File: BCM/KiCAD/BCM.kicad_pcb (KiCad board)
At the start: 2 copper layers, 150 x 99.1 mm, 157 parts, among them J10 Back_9, J11 Back_10, J12 Back_11, J13 Back_12, J14 Eye1, J15 Eye2, J16 Nose, J17 S1, J18 S2, J19 S3, J2 Back_1, J20 S4, J21 S5, J22 Door2, J23 Door1, J24 But1, J25 But2, J26 But3, J27 But4, J28 But5, J29 But6, J3 Back_2, J30 Power, J4 Back_3, J5 Back_4, J6 Back_5, J7 Back_6, J8 Back_7, J9 Back_8, Q1 2N7002, Q10 2N7002, Q11 2N7002, Q12 2N7002, Q13 2N7002, Q14 2N7002, Q15 2N7002, Q16 2N7002, Q17 2N7002, Q18 2N7002, Q19 2N7002, Q2 2N7002, Q20 2N7002, Q3 2N7002, Q4 2N7002, Q5 2N7002, Q6 2N7002, Q7 2N7002, Q8 2N7002, Q9 2N7002, U1 TPS54331D

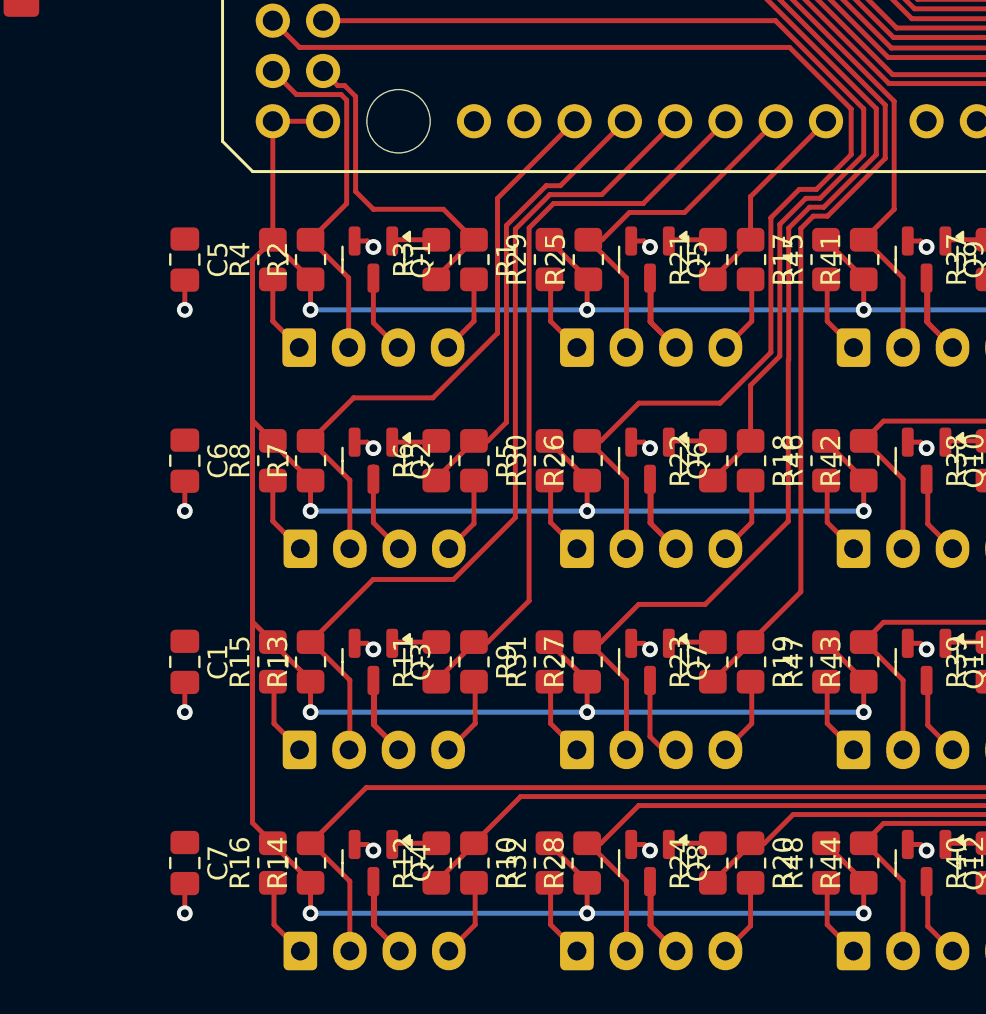
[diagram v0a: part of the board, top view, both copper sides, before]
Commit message: move buttons to own supply rail
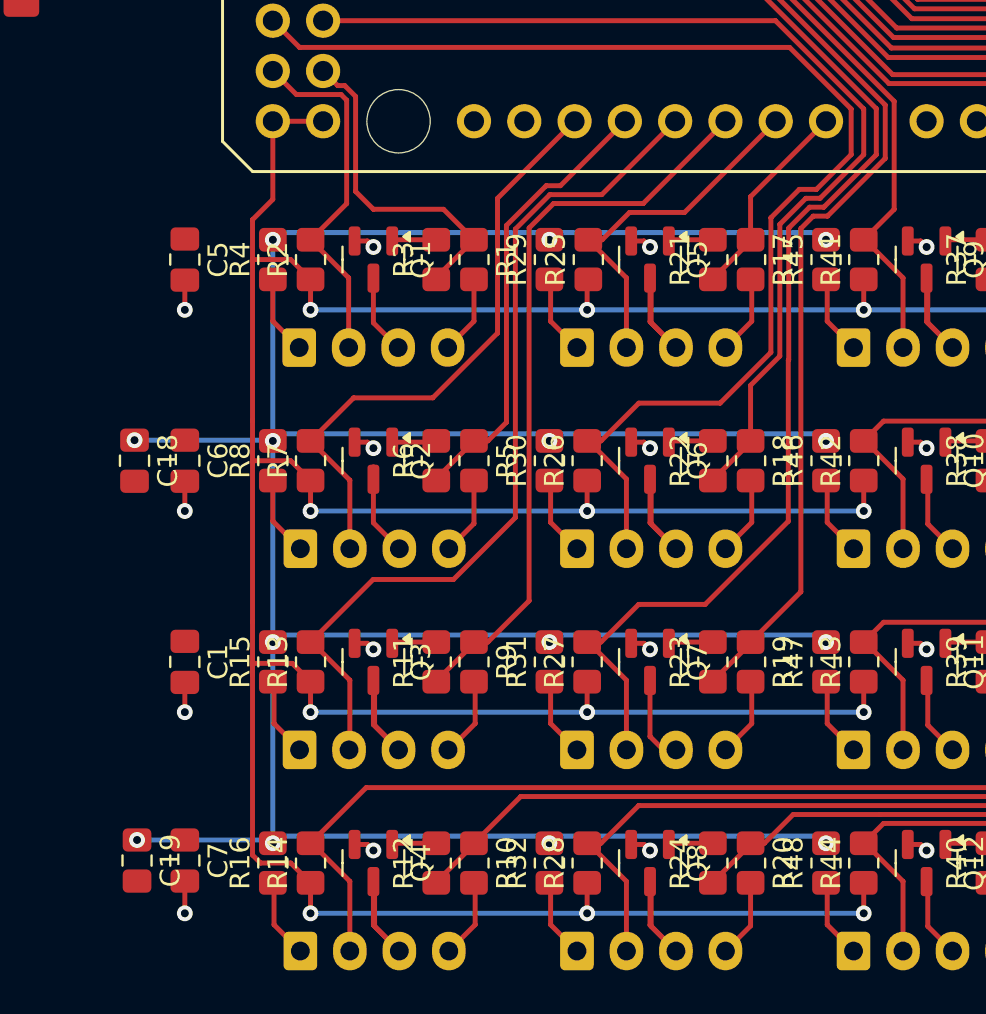
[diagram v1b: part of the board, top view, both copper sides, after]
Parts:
- added C18: C_Small, Capacitor_SMD:C_0805_2012Metric_Pad1.18x1.45mm_HandSolder, F.Cu at (90.8, 99.7)
- added C19: C_Small, Capacitor_SMD:C_0805_2012Metric_Pad1.18x1.45mm_HandSolder, F.Cu at (90.9, 119.9)
- moved C7 0.13 mm to (93.3, 119.9)
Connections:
- R15 pad 2: +5V -> Button +Ve
- R16 pad 2: +5V -> Button +Ve
- R29 pad 2: +5V -> Button +Ve
- R30 pad 2: +5V -> Button +Ve
- R31 pad 2: +5V -> Button +Ve
- R32 pad 2: +5V -> Button +Ve
- R4 pad 2: +5V -> Button +Ve
- R45 pad 2: +5V -> Button +Ve
- R46 pad 2: +5V -> Button +Ve
- R47 pad 2: +5V -> Button +Ve
- R48 pad 2: +5V -> Button +Ve
- R8 pad 2: +5V -> Button +Ve
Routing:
- net Button +Ve: track 0.00 -> 158.6 mm, vias 0 -> 14
- net +5V: track 423.3 -> 402.3 mm
